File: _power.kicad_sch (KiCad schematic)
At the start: 47 parts, among them J6 Power IN, J7 5V_1, J8 5V_2, Q5 HYG210P06LQ1D, U7 XL4001, U8 XL4001

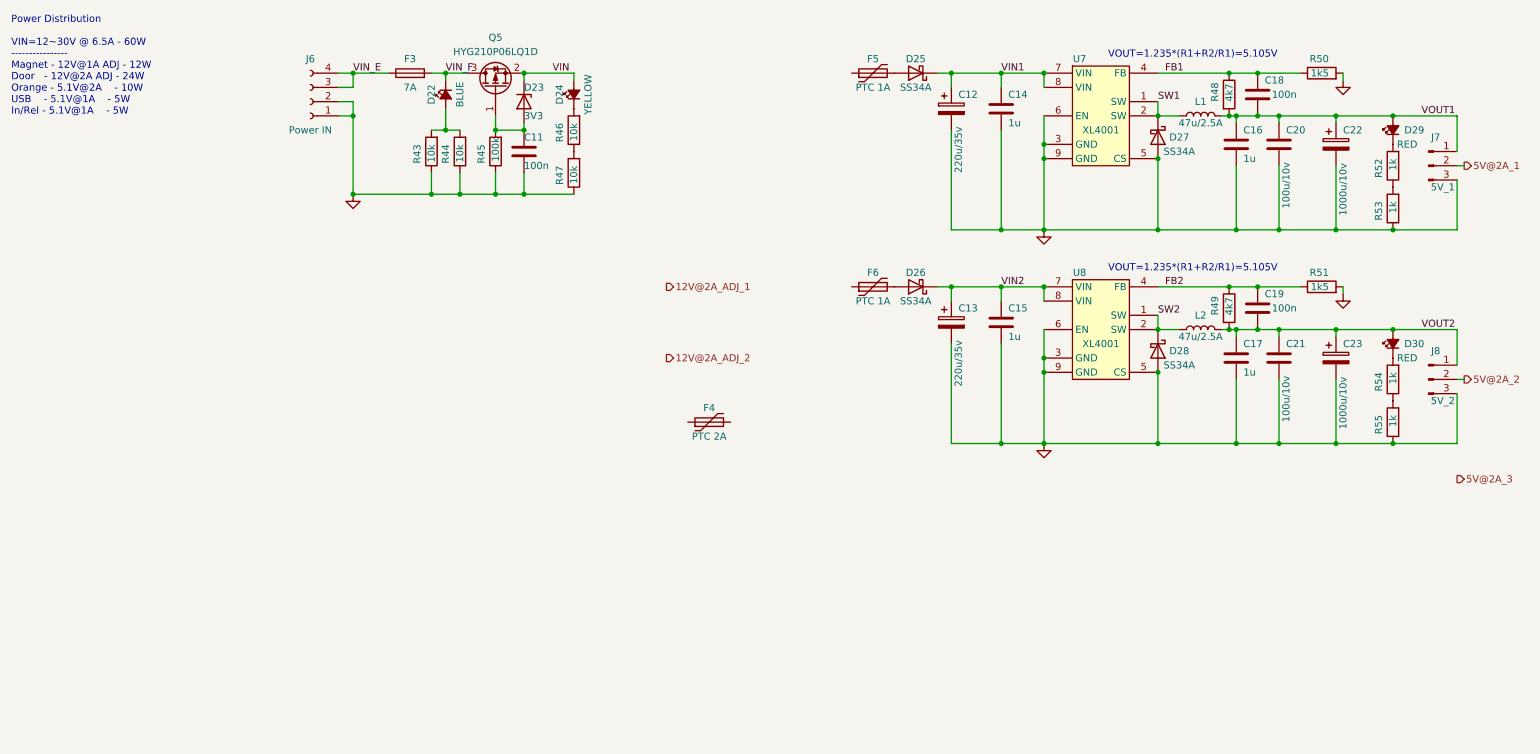
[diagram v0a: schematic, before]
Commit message: most stuff squeezed on board
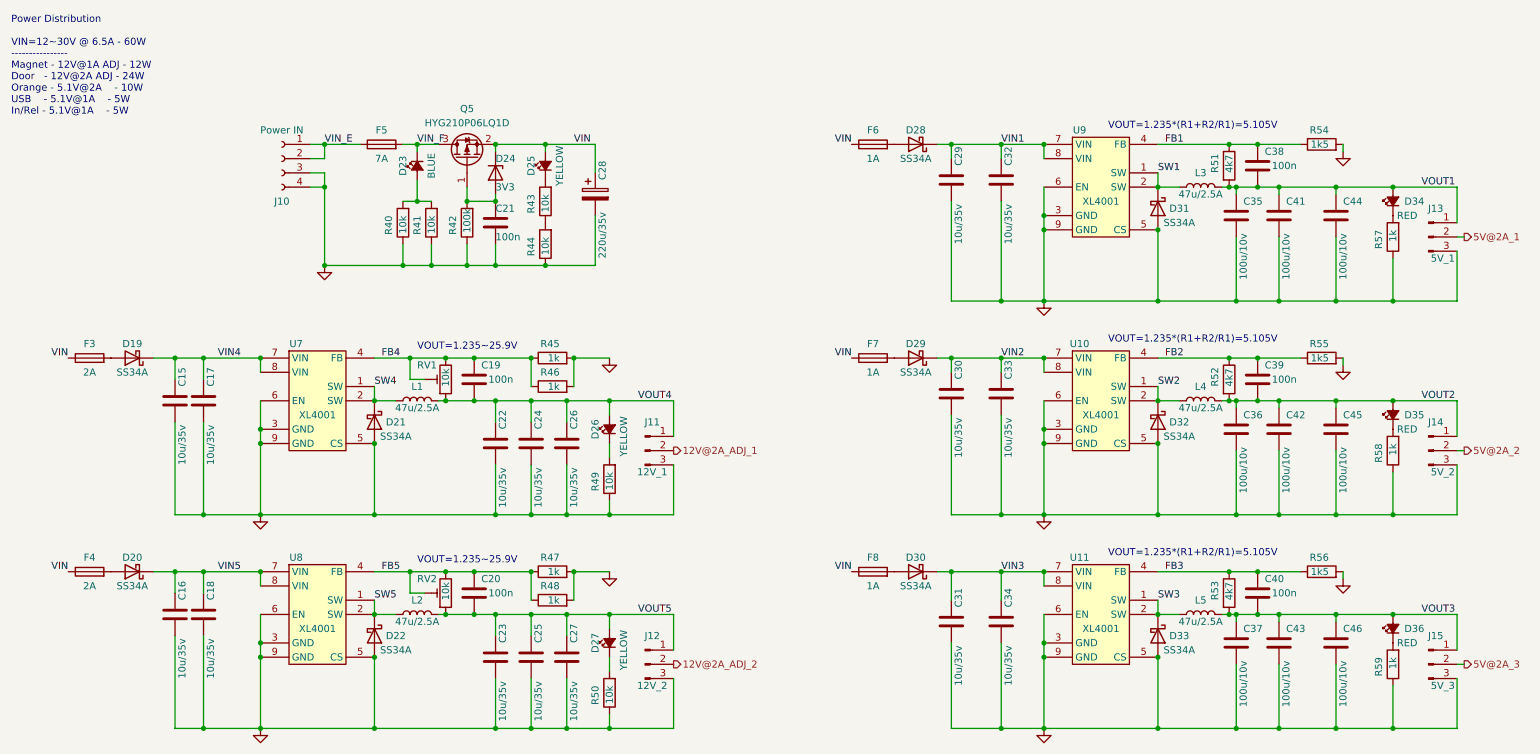
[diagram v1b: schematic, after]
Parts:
- removed C12, C13: 220u/35v, Capacitor_SMD:CP_Elec_10x10, symbol Device:C_Polarized
- removed C14: 1u, Capacitor_SMD:C_0805_2012Metric, symbol Device:C
- removed C22, C23: 1000u/10v, Capacitor_SMD:CP_Elec_10x10, symbol Device:C_Polarized
- removed F6: PTC 1A, -local:Fuse_2920_7451Metric_Pad2.10x5.45mm_HandSolder, symbol Device:Polyfuse
- removed J6: Power IN, TerminalBlock_Phoenix:TerminalBlock_Phoenix_PT-1,5-4-3.5-H_1x04_P3.50mm_Horizontal, symbol Connector:Conn_01x04_Female
- removed R55: 1k, Resistor_SMD:R_0805_2012Metric, symbol Device:R
- added C18, C22, C23, C24, C25, C26, C27, C29, C30, C31, C32, C33, C34: 10u/35v, Capacitor_SMD:C_1206_3216Metric, symbol Device:C
- added C19, C20, C40: 100n, Capacitor_SMD:C_0805_2012Metric, symbol Device:C
- added C28: 220u/35v, Capacitor_SMD:CP_Elec_10x10, symbol Device:C_Polarized
- added C35, C36, C37, C43, C44, C45, C46: 100u/10v, Capacitor_SMD:C_1206_3216Metric, symbol Device:C
- added D19, D20, D21, D22, D30, D33: SS34A, Diode_SMD:D_SMA, symbol Diode:CDBA340-HF
- added D26, D27: YELLOW, LED_SMD:LED_0805_2012Metric_Pad1.15x1.40mm_HandSolder, symbol Device:LED_Small_Filled
- added D36: RED, LED_SMD:LED_0805_2012Metric_Pad1.15x1.40mm_HandSolder, symbol Device:LED_Small_Filled
- added F4: 2A, Fuse:Fuse_1206_3216Metric_Pad1.42x1.75mm_HandSolder, symbol Device:Fuse
- added F7, F8: 1A, Fuse:Fuse_1206_3216Metric_Pad1.42x1.75mm_HandSolder, symbol Device:Fuse
- added J10: Power IN, TerminalBlock_Phoenix:TerminalBlock_Phoenix_PT-1,5-4-3.5-H_1x04_P3.50mm_Horizontal, symbol Connector:Conn_01x04_Female
- added J11: 12V_1, Connector_PinHeader_2.54mm:PinHeader_1x03_P2.54mm_Vertical, symbol Connector:Conn_01x03_Male
- added J12: 12V_2, Connector_PinHeader_2.54mm:PinHeader_1x03_P2.54mm_Vertical, symbol Connector:Conn_01x03_Male
- added J15: 5V_3, Connector_PinHeader_2.54mm:PinHeader_1x03_P2.54mm_Vertical, symbol Connector:Conn_01x03_Male
- added L1, L2, L5: 47u/2.5A, -local:L_12x12mm_H8mm__D11.0_P5.0_universal, symbol Device:L
- added R45, R46, R47, R48, R59: 1k, Resistor_SMD:R_0805_2012Metric, symbol Device:R
- added R49, R50: 10k, Resistor_SMD:R_0805_2012Metric, symbol Device:R
- added R56: 1k5, Resistor_SMD:R_0805_2012Metric, symbol Device:R
- added RV1, RV2: 10k, Potentiometer_THT:Potentiometer_Bourns_3296W_Vertical, symbol Device:R_Potentiometer_Trim
- added U11, U7, U8: XL4001, Package_SO:Texas_HTSOP-8-1EP_3.9x4.9mm_P1.27mm_EP2.95x4.9mm_Mask2.4x3.1mm_ThermalVias, symbol -xlsemi:XL4001
- C15, C16, C17: value 1u -> 10u/35v; footprint Capacitor_SMD:C_0805_2012Metric -> Capacitor_SMD:C_1206_3216Metric; LCSC Part Number C126592 -> C92797; WE (none) -> 885012108022
- F3: renamed from F4; value PTC 2A -> 2A; footprint -local:Fuse_2920_7451Metric_Pad2.10x5.45mm_HandSolder -> Fuse:Fuse_1206_3216Metric_Pad1.42x1.75mm_HandSolder; symbol Device:Polyfuse -> Device:Fuse; LCSC Part Number C910843 -> C187595
- F5: renamed from F3; footprint (none) -> Inductor_SMD:L_1206_3216Metric_Pad1.42x1.75mm_HandSolder; LCSC Part Number (none) -> C136352; WE (none) -> C136352
- F6: renamed from F5; value PTC 1A -> 1A; footprint -local:Fuse_2920_7451Metric_Pad2.10x5.45mm_HandSolder -> Fuse:Fuse_1206_3216Metric_Pad1.42x1.75mm_HandSolder; symbol Device:Polyfuse -> Device:Fuse; LCSC Part Number C409807 -> C151135
- J13: renamed from J7; footprint (none) -> Connector_PinHeader_2.54mm:PinHeader_1x03_P2.54mm_Vertical
- J14: renamed from J8; footprint (none) -> Connector_PinHeader_2.54mm:PinHeader_1x03_P2.54mm_Vertical
- L3: renamed from L1; value 47u/2.5A -> 47u/2.5A
- L4: renamed from L2; value 47u/2.5A -> 47u/2.5A
- R53: value 1k -> 4k7
- renumbered C11 to C21, C18 to C38, C19 to C39, C20 to C41, C21 to C42, D22 to D23, D23 to D24, D24 to D25, D25 to D28, D26 to D29, D27 to D31, D28 to D32, D29 to D34, D30 to D35, R43 to R40, R44 to R41, R45 to R42, R46 to R43, R47 to R44, R48 to R51, R49 to R52, R50 to R54, R51 to R55, R52 to R57, R54 to R58, U8 to U10, U7 to U9
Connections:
- net 12V@2A_ADJ_1: now also J11.2 (Pin_2)
- net 12V@2A_ADJ_2: now also J12.2 (Pin_2)
- net 5V@2A_3: now also J15.2 (Pin_2)
- net GND: now also R57.1, R58.1, C18.2, C22.2, C23.2, C24.2, C25.2, C26.2, C27.2, C28.2, C29.2, C30.2, C31.2, C32.2, C33.2, C34.2, C35.2, C36.2, C37.2, C43.2, C44.2, C45.2, C46.2, D21.2 (A), D22.2 (A), D33.2 (A), J10.3 (Pin_3), J10.4 (Pin_4), J11.3 (Pin_3), J12.3 (Pin_3), J15.3 (Pin_3), R45.2, R46.2, R47.2, R48.2, R49.1, R50.1, R56.2, R59.1, U11.3 (GND), U11.5 (CS), U11.6 (EN), U11.9 (GND), U7.3 (GND), U7.5 (CS), U7.6 (EN), U7.9 (GND), U8.3 (GND), U8.5 (CS), U8.6 (EN), U8.9 (GND); no longer R53.1
- net VIN: now also F3.1, F6.1, C28.1, F4.1, F7.1, F8.1
- net VIN1: now also C29.1, C32.1
- net VIN2: now also C30.1, C33.1; no longer C15.1
- net VIN_E: now also J10.1 (Pin_1), J10.2 (Pin_2)
- net VOUT1: now also C35.1, C44.1; no longer C16.1
- net VOUT2: now also C36.1, C45.1; no longer C17.1
- net VOUT3: now reaches R53.2
- net VOUT3: now also C37.1, C40.2, C43.1, C46.1, D36.2 (A), J15.1 (Pin_1), L5.2; no longer R57.1
- net at F3.2: now also D19.2 (A)
- net at D29.2 (A): now also F7.2
- new net: D30.2 (A), F8.2
- new net: D26.1 (K), R49.2
- new net: D27.1 (K), R50.2
- new net: D20.2 (A), F4.2
- new net: D36.1 (K), R59.2
- new net FB3: C40.1, R53.1, R56.1, U11.4 (FB)
- new net FB4: C19.1, R45.1, R46.1, RV1.2, RV1.3, U7.4 (FB)
- new net FB5: C20.1, R47.1, R48.1, RV2.2, RV2.3, U8.4 (FB)
- new net SW3: D33.1 (K), L5.1, U11.1 (SW), U11.2 (SW)
- new net SW4: D21.1 (K), L1.1, U7.1 (SW), U7.2 (SW)
- new net SW5: D22.1 (K), L2.1, U8.1 (SW), U8.2 (SW)
- new net VIN3: C31.1, C34.1, D30.1 (K), U11.7 (VIN), U11.8 (VIN)
- new net VIN4: C15.1, C17.1, D19.1 (K), U7.7 (VIN), U7.8 (VIN)
- new net VIN5: C16.1, C18.1, D20.1 (K), U8.7 (VIN), U8.8 (VIN)
- new net VOUT4: C19.2, C22.1, C24.1, C26.1, D26.2 (A), J11.1 (Pin_1), L1.2, RV1.1
- new net VOUT5: C20.2, C23.1, C25.1, C27.1, D27.2 (A), J12.1 (Pin_1), L2.2, RV2.1
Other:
- note added: "VOUT=1.235~25.9V"
- moved on the sheet: C21, C38, C39, C41, C42, D23, D24, D25, D28, D29, D31, D32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
